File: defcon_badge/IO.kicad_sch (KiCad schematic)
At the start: 9 parts, among them J30 SAO 2x3, J31 microSD, SW20 TS-1187A, SW21 TS-1187A, SW22 TS-1187A, SW23 TS-1187A

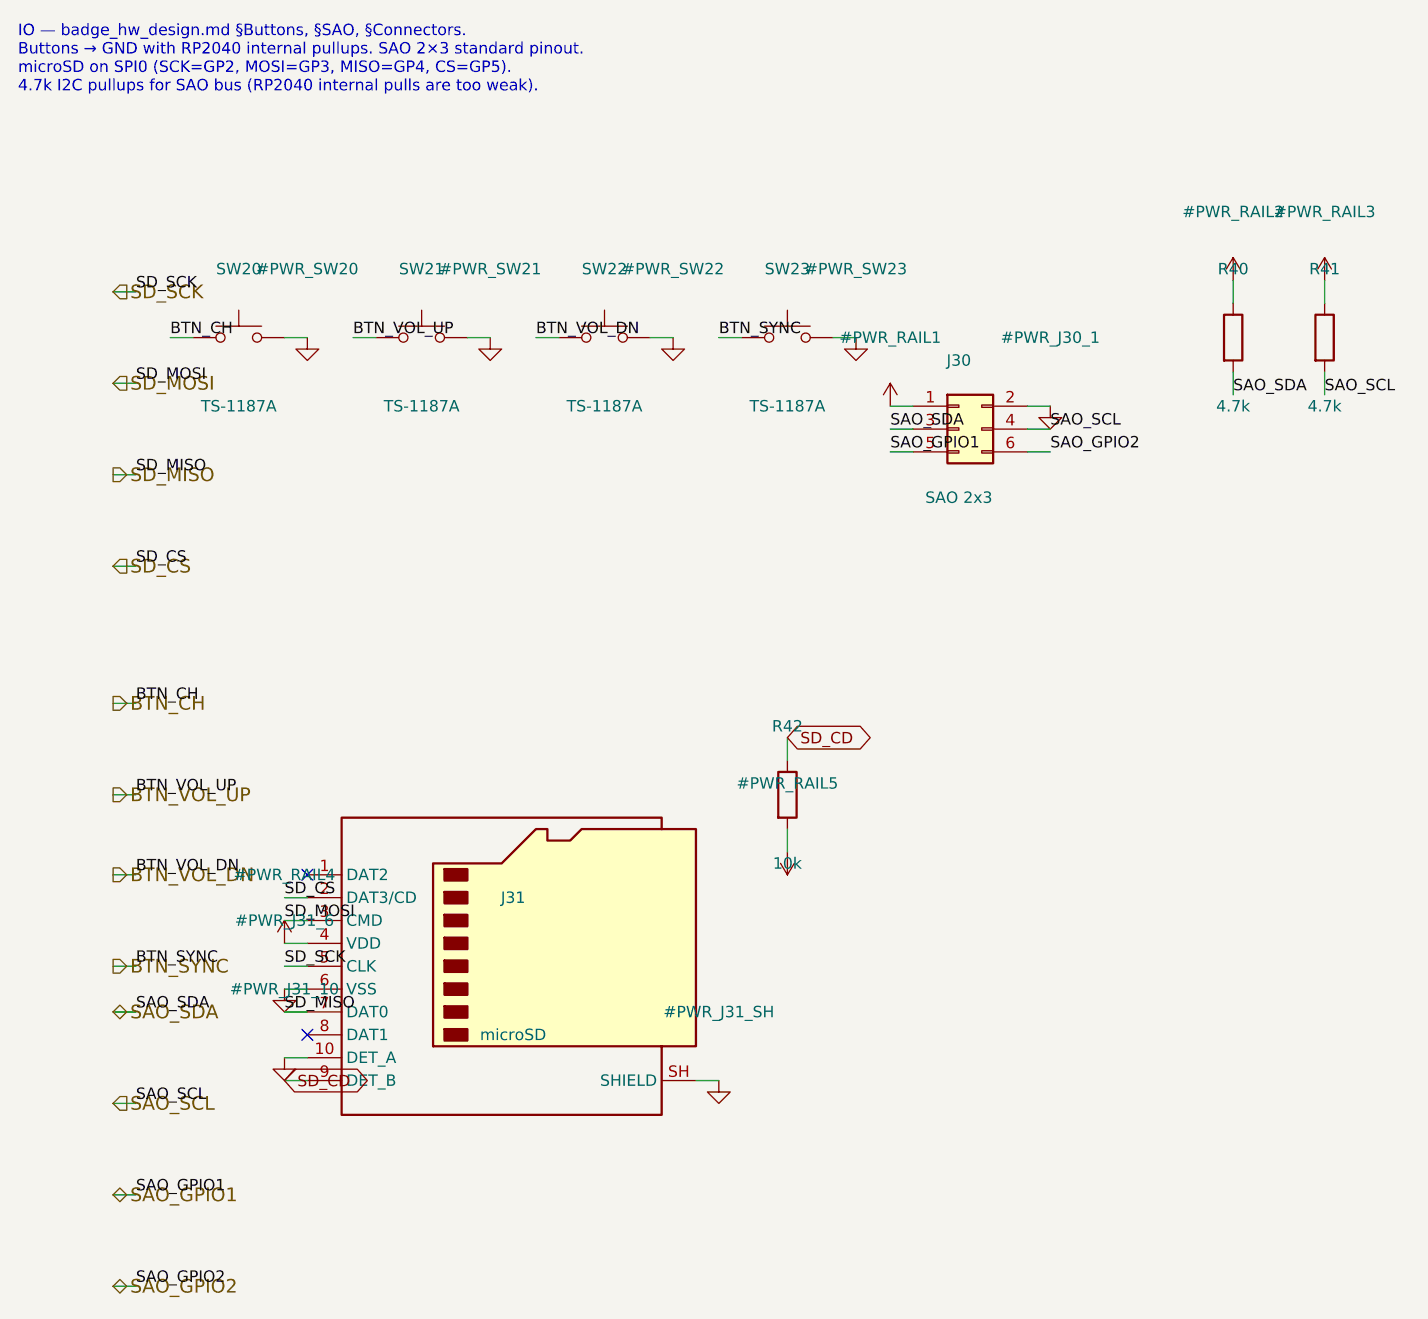
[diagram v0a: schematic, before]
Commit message: Routing redo
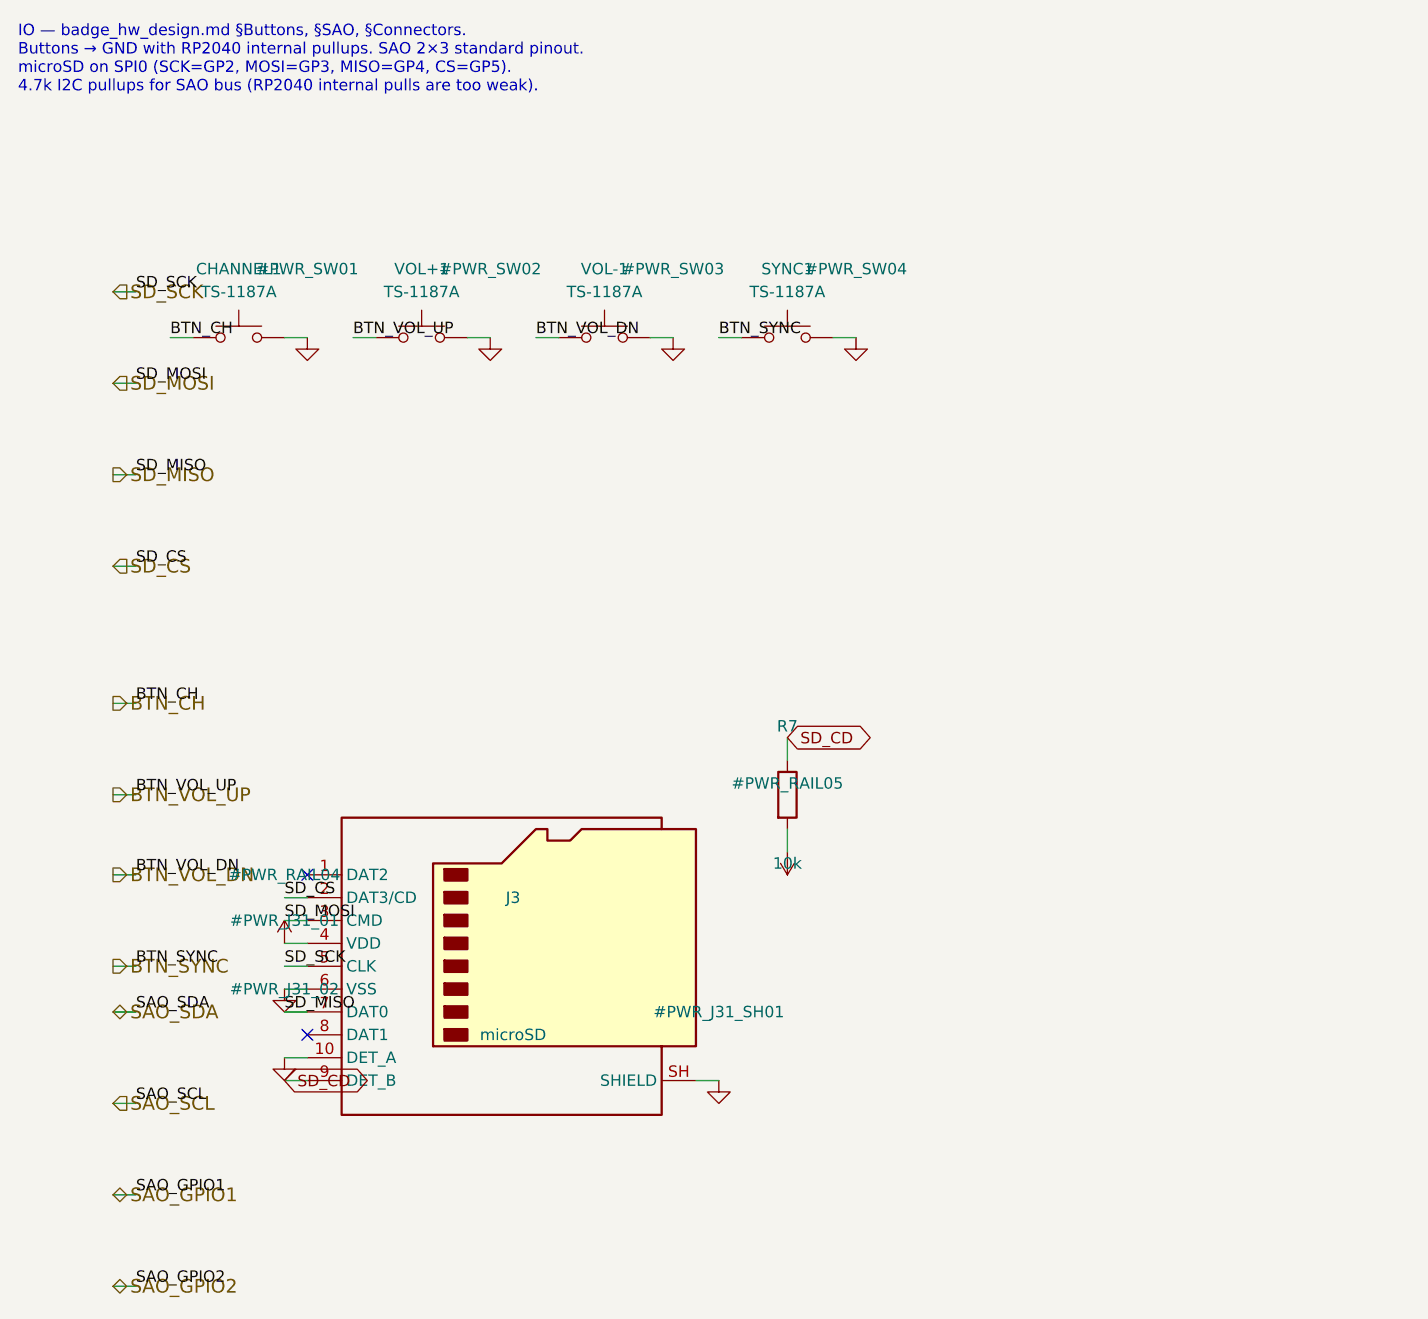
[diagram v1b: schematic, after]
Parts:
- removed J30: SAO 2x3, Connector_PinHeader_2.54mm:PinHeader_2x03_P2.54mm_Vertical, symbol Connector_Generic:Conn_02x03_Odd_Even
- removed R40, R41: 4.7k, Resistor_SMD:R_0402_1005Metric, symbol Device:R
- renumbered SW20 to CHANNEL1, J31 to J3, R42 to R7, SW23 to SYNC1, SW21 to VOL+1, SW22 to VOL-1
